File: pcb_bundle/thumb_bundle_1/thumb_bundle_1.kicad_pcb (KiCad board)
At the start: 2 copper layers, 102 x 107.3 mm, 42 parts

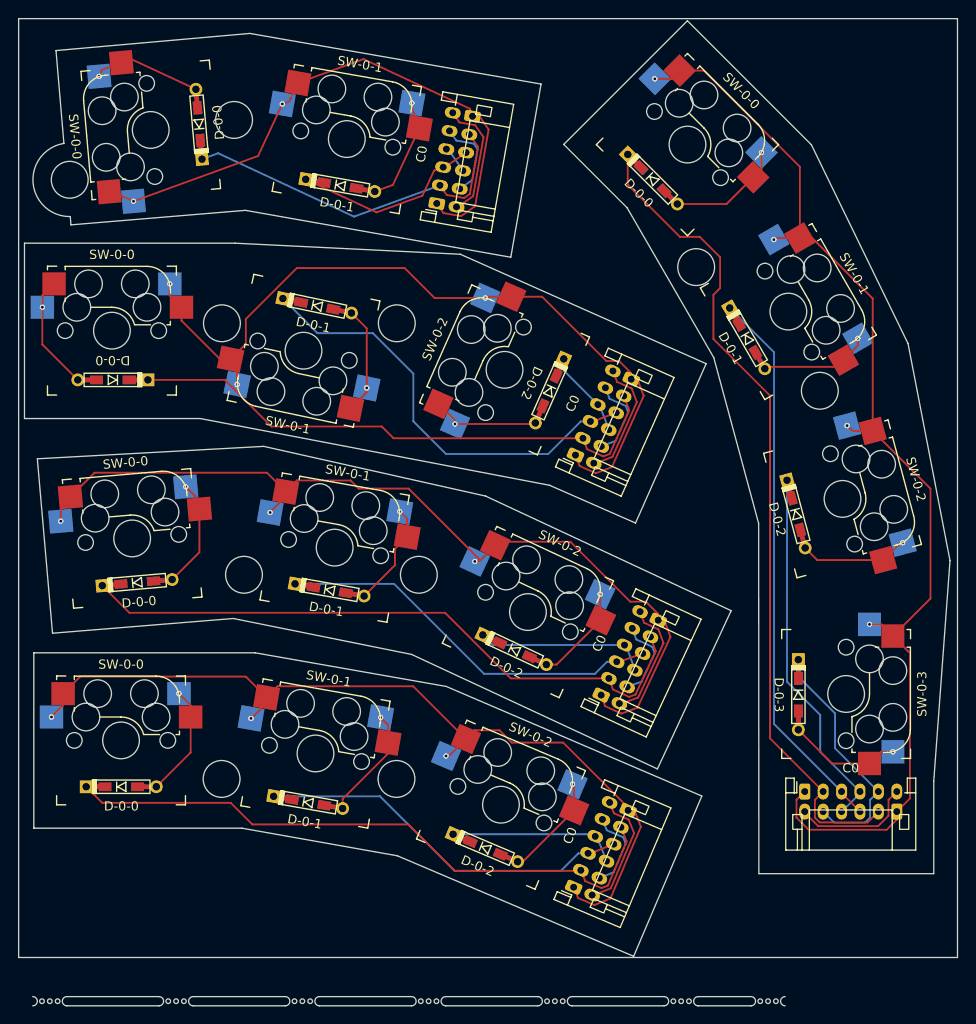
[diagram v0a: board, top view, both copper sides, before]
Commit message: net synced and gerber created
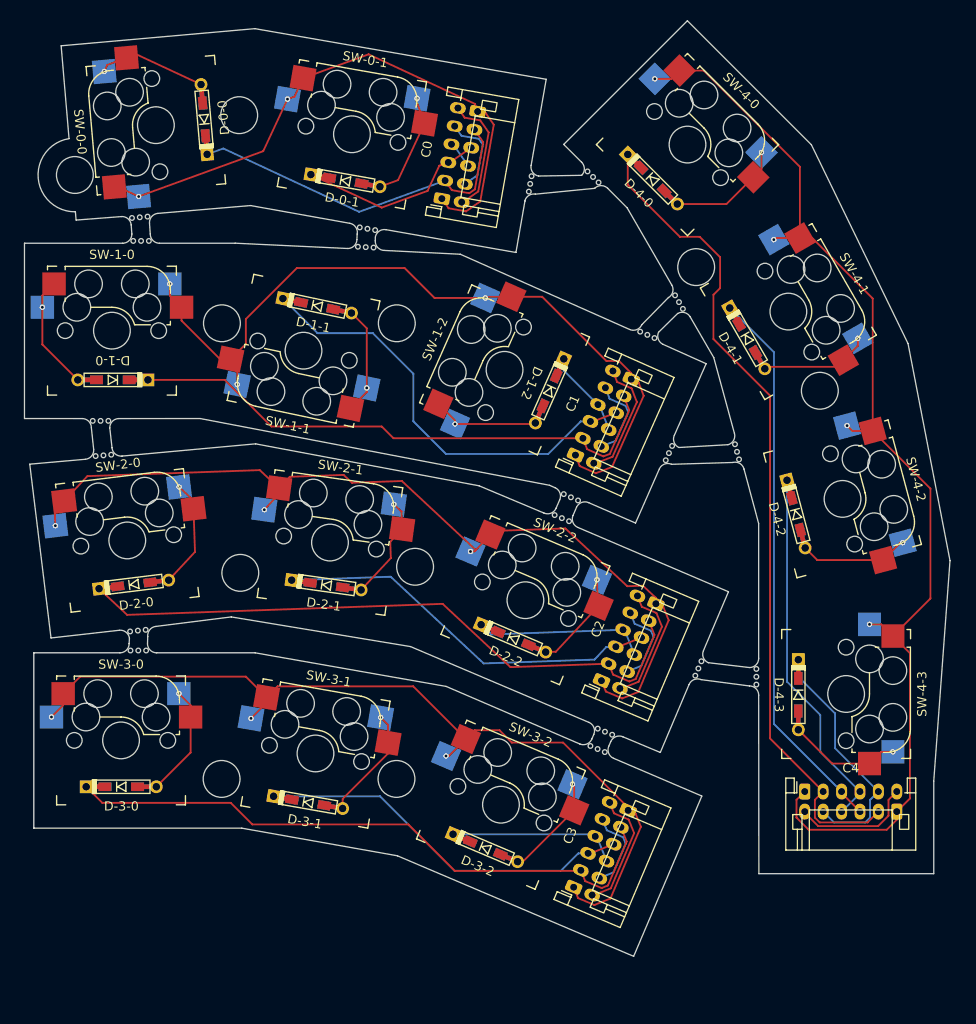
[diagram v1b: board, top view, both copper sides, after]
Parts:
- removed mouse-bite-1mm-3mm (x7): VAL**, Panelization:BreakLine_3h_D0.5mm_P0.85mm
- added REF**: MouseBite-Part_2.0x2.0mm_outset_D0.5mm_P0.85mm_3h, Panelization:MouseBite-Part_2.0x2.0mm_outset_D0.5mm_P0.85mm_3h, F.Cu at (55.2, 111.9)
- added REF**: MouseBite-Part_2.0x2.0mm_outset_D0.5mm_P0.85mm_3h, Panelization:MouseBite-Part_2.0x2.0mm_outset_D0.5mm_P0.85mm_3h, F.Cu at (101.2, 100.2)
- added REF**: MouseBite-Part_2.0x2.0mm_outset_D0.5mm_P0.85mm_3h, Panelization:MouseBite-Part_2.0x2.0mm_outset_D0.5mm_P0.85mm_3h, F.Cu at (80.0, 70.8)
- added REF**: MouseBite-Part_2.0x2.0mm_outset_D0.5mm_P0.85mm_3h, Panelization:MouseBite-Part_2.0x2.0mm_outset_D0.5mm_P0.85mm_3h, F.Cu at (120.6, 92.7)
- added REF**: MouseBite-Part_2.0x2.0mm_outset_D0.5mm_P0.85mm_3h, Panelization:MouseBite-Part_2.0x2.0mm_outset_D0.5mm_P0.85mm_3h, F.Cu at (104.9, 62.7)
- added REF**: MouseBite-Part_2.0x2.0mm_outset_D0.5mm_P0.85mm_3h, Panelization:MouseBite-Part_2.0x2.0mm_outset_D0.5mm_P0.85mm_3h, F.Cu at (55.4, 67.0)
- added REF**: MouseBite-Part_2.0x2.0mm_outset_D0.5mm_P0.85mm_3h, Panelization:MouseBite-Part_2.0x2.0mm_outset_D0.5mm_P0.85mm_3h, F.Cu at (55.3, 114.6)
- added REF**: MouseBite-Part_2.0x2.0mm_outset_D0.5mm_P0.85mm_3h, Panelization:MouseBite-Part_2.0x2.0mm_outset_D0.5mm_P0.85mm_3h, F.Cu at (122.7, 117.2)
- added REF**: MouseBite-Part_2.0x2.0mm_outset_D0.5mm_P0.85mm_3h, Panelization:MouseBite-Part_2.0x2.0mm_outset_D0.5mm_P0.85mm_3h, F.Cu at (102.4, 97.5)
- added REF**: MouseBite-Part_2.0x2.0mm_outset_D0.5mm_P0.85mm_3h, Panelization:MouseBite-Part_2.0x2.0mm_outset_D0.5mm_P0.85mm_3h, F.Cu at (51.2, 89.2)
- added REF**: MouseBite-Part_2.0x2.0mm_outset_D0.5mm_P0.85mm_3h, Panelization:MouseBite-Part_2.0x2.0mm_outset_D0.5mm_P0.85mm_3h, F.Cu at (51.5, 93.4)
- added REF**: MouseBite-Part_2.0x2.0mm_outset_D0.5mm_P0.85mm_3h, Panelization:MouseBite-Part_2.0x2.0mm_outset_D0.5mm_P0.85mm_3h, F.Cu at (106.1, 122.9)
- added REF**: MouseBite-Part_2.0x2.0mm_outset_D0.5mm_P0.85mm_3h, Panelization:MouseBite-Part_2.0x2.0mm_outset_D0.5mm_P0.85mm_3h, F.Cu at (110.5, 80.3)
- added REF**: MouseBite-Part_2.0x2.0mm_outset_D0.5mm_P0.85mm_3h, Panelization:MouseBite-Part_2.0x2.0mm_outset_D0.5mm_P0.85mm_3h, F.Cu at (97.6, 63.6)
- added REF**: MouseBite-Part_2.0x2.0mm_outset_D0.5mm_P0.85mm_3h, Panelization:MouseBite-Part_2.0x2.0mm_outset_D0.5mm_P0.85mm_3h, F.Cu at (115.9, 116.2)
- added REF**: MouseBite-Part_2.0x2.0mm_outset_D0.5mm_P0.85mm_3h, Panelization:MouseBite-Part_2.0x2.0mm_outset_D0.5mm_P0.85mm_3h, F.Cu at (105.1, 125.3)
- added REF**: MouseBite-Part_2.0x2.0mm_outset_D0.5mm_P0.85mm_3h, Panelization:MouseBite-Part_2.0x2.0mm_outset_D0.5mm_P0.85mm_3h, F.Cu at (55.6, 70.1)
- added REF**: MouseBite-Part_2.0x2.0mm_outset_D0.5mm_P0.85mm_3h, Panelization:MouseBite-Part_2.0x2.0mm_outset_D0.5mm_P0.85mm_3h, F.Cu at (80.2, 68.3)
- added REF**: MouseBite-Part_2.0x2.0mm_outset_D0.5mm_P0.85mm_3h, Panelization:MouseBite-Part_2.0x2.0mm_outset_D0.5mm_P0.85mm_3h, F.Cu at (112.7, 92.8)
- added REF**: MouseBite-Part_2.0x2.0mm_outset_D0.5mm_P0.85mm_3h, Panelization:MouseBite-Part_2.0x2.0mm_outset_D0.5mm_P0.85mm_3h, F.Cu at (114.3, 76.4)
- moved C2 1.57 mm to (105.6, 117.6), turned to 67 degrees
- moved SW-2-2 1.32 mm to (97.4, 108.9), turned to -23 degrees
- moved D-2-2 1.25 mm to (96.1, 113.0), turned to -23 degrees
- moved D-0-1 0.76 mm to (77.8, 63.3)
- moved SW-0-0 0.76 mm to (57.2, 57.3)
- moved C0 0.76 mm to (88.3, 65.3)
- moved D-0-0 0.76 mm to (62.4, 56.6)
- moved SW-0-1 0.76 mm to (78.5, 58.3)
- moved SW-2-1 0.75 mm to (76.1, 102.6), turned to -8 degrees
- moved D-2-1 0.64 mm to (75.7, 107.2), turned to -8 degrees
- moved SW-2-0 0.57 mm to (54.1, 102.4), turned to 7 degrees
- moved D-2-0 0.41 mm to (54.8, 107.2), turned to 7 degrees
- renumbered C0 to C1, C0 to C2, C0 to C3, C0 to C4, D-0-0 to D-1-0, D-0-1 to D-1-1, D-0-2 to D-1-2, D-0-0 to D-2-0, D-0-1 to D-2-1, D-0-2 to D-2-2, D-0-0 to D-3-0, D-0-1 to D-3-1, D-0-2 to D-3-2, D-0-0 to D-4-0, D-0-1 to D-4-1, D-0-2 to D-4-2, D-0-3 to D-4-3, SW-0-0 to SW-1-0, SW-0-1 to SW-1-1, SW-0-2 to SW-1-2, SW-0-0 to SW-2-0, SW-0-1 to SW-2-1, SW-0-2 to SW-2-2, SW-0-0 to SW-3-0, SW-0-1 to SW-3-1, SW-0-2 to SW-3-2, SW-0-0 to SW-4-0, SW-0-1 to SW-4-1, SW-0-2 to SW-4-2, SW-0-3 to SW-4-3
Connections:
- C1 pad 1: COL0 -> COL1
- C1 pad 2: ROW0-0 -> ROW0-1
- C1 pad 3: ROW1-0 -> ROW1-1
- C1 pad 4: ROW2-0 -> ROW2-1
- C1 pad 5: ROW3-0 -> ROW3-1
- C1 pad 6: ROW4-0 -> ROW4-1
- C2 pad 1: COL0 -> COL2
- C2 pad 2: ROW0-0 -> ROW0-2
- C2 pad 3: ROW1-0 -> ROW1-2
- C2 pad 4: ROW2-0 -> ROW2-2
- C2 pad 5: ROW3-0 -> ROW3-2
- C2 pad 6: ROW4-0 -> ROW4-2
- C3 pad 1: COL0 -> COL3
- C3 pad 2: ROW0-0 -> ROW0-3
- C3 pad 3: ROW1-0 -> ROW1-3
- C3 pad 4: ROW2-0 -> ROW2-3
- C3 pad 5: ROW3-0 -> ROW3-3
- C3 pad 6: ROW4-0 -> ROW4-3
- C4 pad 1: COL0 -> COL4
- C4 pad 2: ROW0-0 -> ROW0-4
- C4 pad 3: ROW1-0 -> ROW1-4
- C4 pad 4: ROW2-0 -> ROW2-4
- C4 pad 5: ROW3-0 -> ROW3-4
- C4 pad 6: ROW4-0 -> ROW4-4
- D-1-0 pad 1: ROW0-0 -> ROW0-1
- D-1-0 pad 2: Net-(D-0-0-A) -> Net-(D-1-0-A)
- D-1-1 pad 1: ROW1-0 -> ROW1-1
- D-1-1 pad 2: Net-(D-0-1-A) -> Net-(D-1-1-A)
- D-1-2 pad 1: ROW2-0 -> ROW2-1
- D-1-2 pad 2: Net-(D-0-2-A) -> Net-(D-1-2-A)
- D-2-0 pad 1: ROW0-0 -> ROW0-2
- D-2-0 pad 2: Net-(D-0-0-A) -> Net-(D-2-0-A)
- D-2-1 pad 1: ROW1-0 -> ROW1-2
- D-2-1 pad 2: Net-(D-0-1-A) -> Net-(D-2-1-A)
- D-2-2 pad 1: ROW2-0 -> ROW2-2
- D-2-2 pad 2: Net-(D-0-2-A) -> Net-(D-2-2-A)
- D-3-0 pad 1: ROW0-0 -> ROW0-3
- D-3-0 pad 2: Net-(D-0-0-A) -> Net-(D-3-0-A)
- D-3-1 pad 1: ROW1-0 -> ROW1-3
- D-3-1 pad 2: Net-(D-0-1-A) -> Net-(D-3-1-A)
- D-3-2 pad 1: ROW2-0 -> ROW2-3
- D-3-2 pad 2: Net-(D-0-2-A) -> Net-(D-3-2-A)
- D-4-0 pad 1: ROW0-0 -> ROW0-4
- D-4-0 pad 2: Net-(D-0-0-A) -> Net-(D-4-0-A)
- D-4-1 pad 1: ROW1-0 -> ROW1-4
- D-4-1 pad 2: Net-(D-0-1-A) -> Net-(D-4-1-A)
- D-4-2 pad 1: ROW2-0 -> ROW2-4
- D-4-2 pad 2: Net-(D-0-2-A) -> Net-(D-4-2-A)
- D-4-3 pad 1: ROW3-0 -> ROW3-4
- SW-1-0 pad 1: Net-(D-0-0-A) -> Net-(D-1-0-A)
- SW-1-0 pad 2: COL0 -> COL1
- SW-1-1 pad 1: Net-(D-0-1-A) -> Net-(D-1-1-A)
- SW-1-1 pad 2: COL0 -> COL1
- SW-1-2 pad 1: Net-(D-0-2-A) -> Net-(D-1-2-A)
- SW-1-2 pad 2: COL0 -> COL1
- SW-2-0 pad 1: Net-(D-0-0-A) -> Net-(D-2-0-A)
- SW-2-0 pad 2: COL0 -> COL2
- SW-2-1 pad 1: Net-(D-0-1-A) -> Net-(D-2-1-A)
- SW-2-1 pad 2: COL0 -> COL2
- SW-2-2 pad 1: Net-(D-0-2-A) -> Net-(D-2-2-A)
- SW-2-2 pad 2: COL0 -> COL2
- SW-3-0 pad 1: Net-(D-0-0-A) -> Net-(D-3-0-A)
- SW-3-0 pad 2: COL0 -> COL3
- SW-3-1 pad 1: Net-(D-0-1-A) -> Net-(D-3-1-A)
- SW-3-1 pad 2: COL0 -> COL3
- SW-3-2 pad 1: Net-(D-0-2-A) -> Net-(D-3-2-A)
- SW-3-2 pad 2: COL0 -> COL3
- SW-4-0 pad 1: Net-(D-0-0-A) -> Net-(D-4-0-A)
- SW-4-0 pad 2: COL0 -> COL4
- SW-4-1 pad 1: Net-(D-0-1-A) -> Net-(D-4-1-A)
- SW-4-1 pad 2: COL0 -> COL4
- SW-4-2 pad 1: Net-(D-0-2-A) -> Net-(D-4-2-A)
- SW-4-2 pad 2: COL0 -> COL4
- SW-4-3 pad 2: COL0 -> COL4
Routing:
- net COL0: track 466.6 -> 63.7 mm, vias 15 -> 2
- net ROW0-0: track 328.6 -> 38.9 mm
- net ROW1-0: track 212.3 -> 20.7 mm
- net COL4: track 0.00 -> 125.2 mm, vias 0 -> 4
- net COL2: track 0.00 -> 97.3 mm, vias 0 -> 3
- net COL3: track 0.00 -> 95.1 mm, vias 0 -> 3
- net ROW0-4: track 0.00 -> 90.7 mm
- net ROW2-0: track 89.1 -> 2.83 mm
- net COL1: track 0.00 -> 85.3 mm, vias 0 -> 3
- net ROW0-2: track 0.00 -> 70.0 mm
- net ROW0-3: track 0.00 -> 68.4 mm
- net ROW0-1: track 0.00 -> 60.7 mm
- net ROW1-4: track 0.00 -> 60.4 mm
- net ROW3-0: track 63.0 -> 9.01 mm
- net ROW4-0: track 65.9 -> 13.2 mm
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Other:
- board size 102 x 107.3 mm -> 100.6 x 101.6 mm
